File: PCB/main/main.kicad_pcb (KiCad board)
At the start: 2 copper layers, 4 parts, among them J1 Conn_01x33_Female, J2 Conn_01x33_Female, J3 Conn_01x33_Female, J4 Conn_01x33_Female

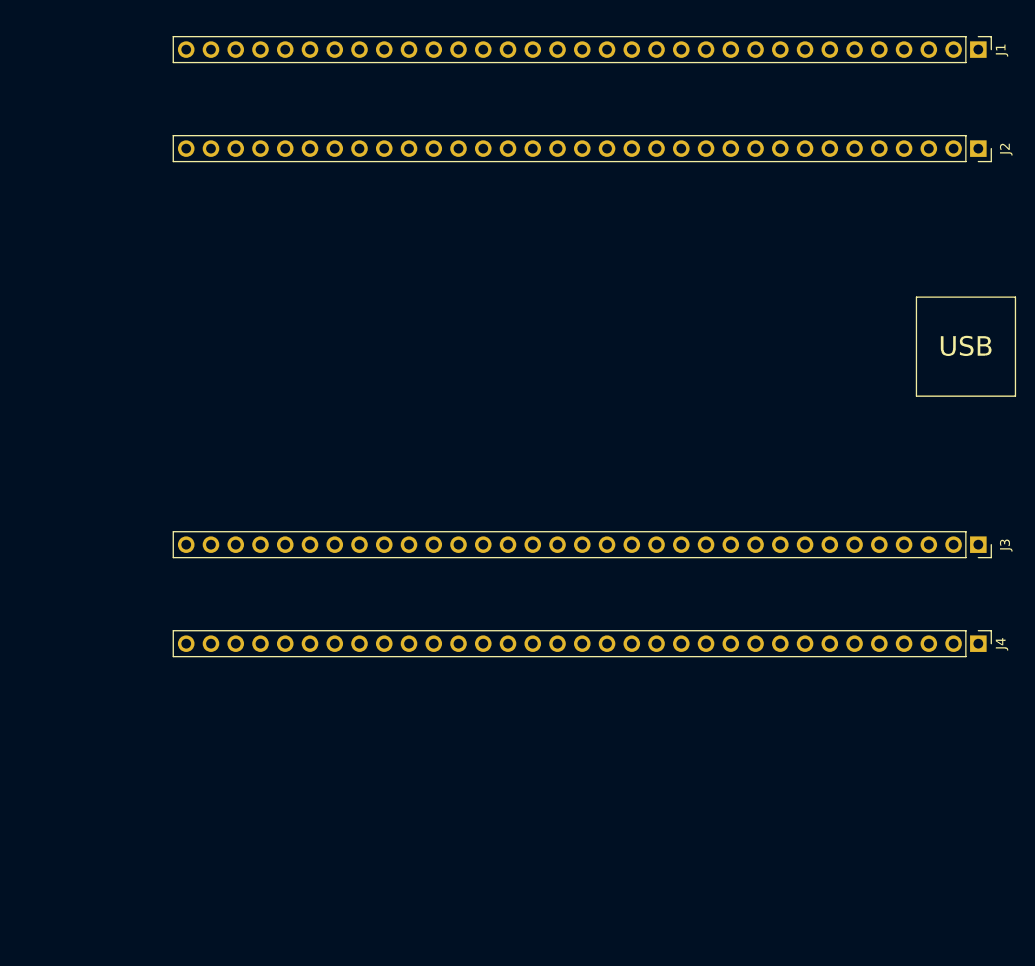
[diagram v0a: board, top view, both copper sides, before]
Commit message: layout started
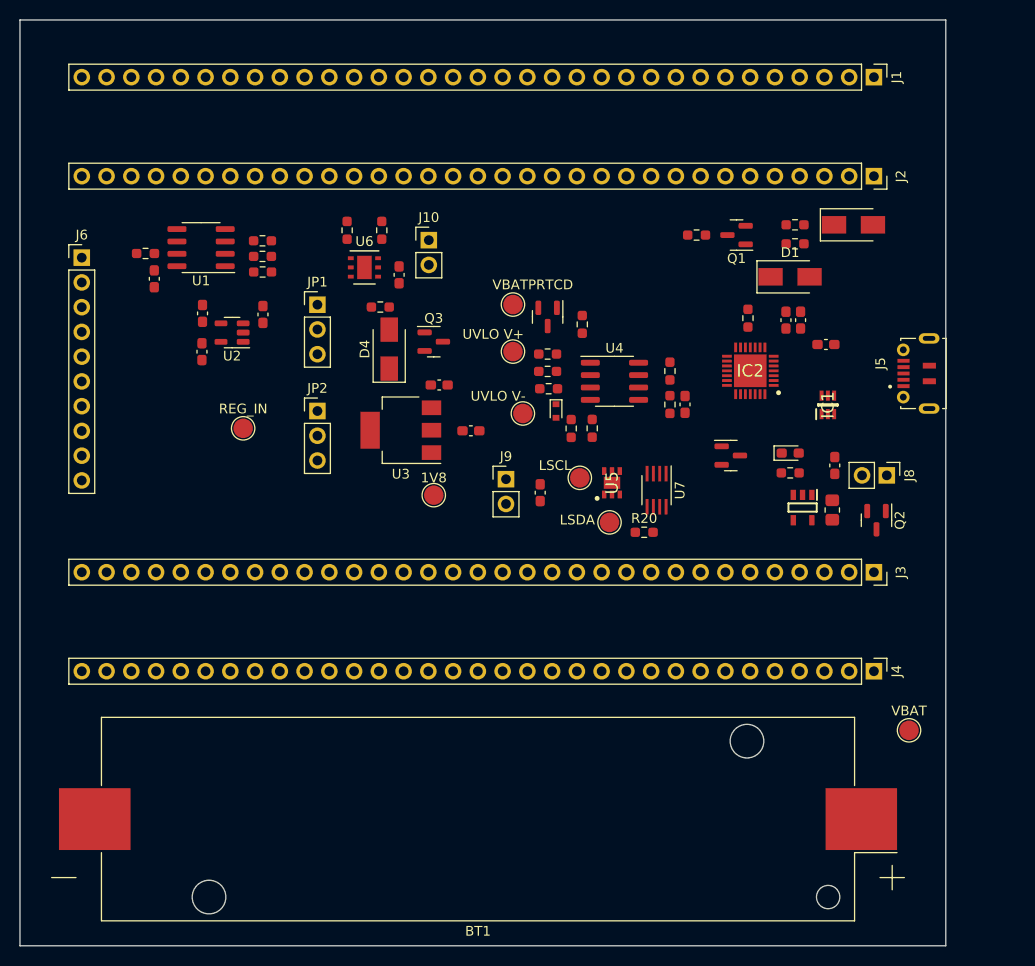
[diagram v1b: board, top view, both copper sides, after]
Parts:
- added 1V8: 1V8, TestPoint:TestPoint_Pad_D2.0mm, F.Cu at (124.5, 111.8)
- added BT1: Battery_Cell, Battery:BatteryHolder_Keystone_1042_1x18650, F.Cu at (129.0, 145.0)
- added C1: 1uF, Capacitor_SMD:C_0603_1608Metric_Pad1.08x0.95mm_HandSolder, F.Cu at (160.6, 93.8)
- added C10: 1uF, Capacitor_SMD:C_0603_1608Metric_Pad1.08x0.95mm_HandSolder, F.Cu at (165.6, 108.7)
- added C11: 1uF, Capacitor_SMD:C_0603_1608Metric_Pad1.08x0.95mm_HandSolder, F.Cu at (150.2, 102.4)
- added C12: 100nF, Capacitor_SMD:C_0603_1608Metric_Pad1.08x0.95mm_HandSolder, F.Cu at (135.4, 111.5)
- added C13: 100nF, Capacitor_SMD:C_0603_1608Metric_Pad1.08x0.95mm_HandSolder, F.Cu at (120.9, 89.2)
- added C2: 100nF, Capacitor_SMD:C_0603_1608Metric_Pad1.08x0.95mm_HandSolder, F.Cu at (162.1, 93.8)
- added C3: 100nF, Capacitor_SMD:C_0603_1608Metric_Pad1.08x0.95mm_HandSolder, F.Cu at (164.7, 96.3)
- added C4: 100nF, Capacitor_SMD:C_0603_1608Metric_Pad1.08x0.95mm_HandSolder, F.Cu at (95.8, 89.6)
- added C5: 1uF, Capacitor_SMD:C_0603_1608Metric_Pad1.08x0.95mm_HandSolder, F.Cu at (106.9, 93.2)
- added C6: 1uF, Capacitor_SMD:C_0603_1608Metric_Pad1.08x0.95mm_HandSolder, F.Cu at (125.0, 100.5)
- added C7: 10nF, Capacitor_SMD:C_0603_1608Metric_Pad1.08x0.95mm_HandSolder, F.Cu at (100.7, 93.1)
- added C8: 1uF, Capacitor_SMD:C_0603_1608Metric_Pad1.08x0.95mm_HandSolder, F.Cu at (128.3, 105.2)
- added C9: 1uF, Capacitor_SMD:C_0603_1608Metric_Pad1.08x0.95mm_HandSolder, F.Cu at (100.7, 97.0)
- added D1: D_Schottky, Diode_SMD:D_SMA, F.Cu at (161.0, 89.4)
- added D2: D_Schottky, Diode_SMD:D_SMA, F.Cu at (167.5, 84.0)
- added D3: CHRG, LED_SMD:LED_0603_1608Metric_Pad1.05x0.95mm_HandSolder, F.Cu at (161.0, 107.4)
- added D4: D_Schottky, Diode_SMD:D_SMA, F.Cu at (119.9, 96.8)
- added D5: D_Zener, Diode_SMD:D_SOD-523, F.Cu at (137.0, 103.1)
- added IC1: SMF05CT1G, SMF05CT1G:SOT65P210X110-6N, F.Cu at (164.9, 102.5)
- added IC2: CP2102-GMR, CP2102-GMR:QFN50P500X500X100-29N-D, F.Cu at (156.9, 99.0)
- added IC3: TP4054-42-SOT25-R, TP4054-42-SOT25-R:SOT95P280X100-5N, F.Cu at (162.3, 113.0)
- added J10: Conn_01x02_Male, Connector_PinHeader_2.54mm:PinHeader_1x02_P2.54mm_Vertical, F.Cu at (124.0, 85.6)
- added J5: USB_B_Micro, MICROXNJ:SHOUHAN_MICROXNJ, F.Cu at (177.0, 99.3)
- added J6: Conn_01x10_Male, Connector_PinHeader_2.54mm:PinHeader_1x10_P2.54mm_Vertical, F.Cu at (88.3, 87.4)
- added J8: Conn_01x02_Male, Connector_PinHeader_2.54mm:PinHeader_1x02_P2.54mm_Vertical, F.Cu at (170.9, 109.7)
- added J9: Conn_01x02_Male, Connector_PinHeader_2.54mm:PinHeader_1x02_P2.54mm_Vertical, F.Cu at (131.9, 110.1)
- added JP1: Jumper_3_Open, Connector_PinHeader_2.54mm:PinHeader_1x03_P2.54mm_Vertical, F.Cu at (112.5, 92.2)
- added JP2: Jumper_3_Open, Connector_PinHeader_2.54mm:PinHeader_1x03_P2.54mm_Vertical, F.Cu at (112.5, 103.1)
- added LSCL: GAS_SCL, TestPoint:TestPoint_Pad_D2.0mm, F.Cu at (139.4, 110.0)
- added LSDA: GAS_SDA, TestPoint:TestPoint_Pad_D2.0mm, F.Cu at (142.5, 114.6)
- added Q1: Q_NMOS_GSD, Package_TO_SOT_SMD:SOT-23, F.Cu at (155.5, 85.1)
- added Q2: Q_PMOS_GSD, Package_TO_SOT_SMD:SOT-23, F.Cu at (169.9, 114.3)
- added Q3: Q_PMOS_GSD, Package_TO_SOT_SMD:SOT-23, F.Cu at (124.5, 96.0)
- added Q4: Q_PMOS_GSD, Package_TO_SOT_SMD:SOT-23, F.Cu at (154.9, 107.7)
- added Q5: Q_PMOS_GSD, Package_TO_SOT_SMD:SOT-23, F.Cu at (136.1, 93.5)
- added R1: 4k7, Resistor_SMD:R_0603_1608Metric_Pad0.98x0.95mm_HandSolder, F.Cu at (161.5, 84.0)
- added R10: 4k7, Resistor_SMD:R_0603_1608Metric_Pad0.98x0.95mm_HandSolder, F.Cu at (119.0, 92.5)
- added R11: 5K1, Resistor_SMD:R_0805_2012Metric_Pad1.20x1.40mm_HandSolder, F.Cu at (165.4, 113.3)
- added R12: 2.2M, Resistor_SMD:R_0603_1608Metric_Pad0.98x0.95mm_HandSolder, F.Cu at (148.7, 99.0)
- added R13: 1M, Resistor_SMD:R_0603_1608Metric_Pad0.98x0.95mm_HandSolder, F.Cu at (148.7, 102.5)
- added R14: 300K, Resistor_SMD:R_0603_1608Metric_Pad0.98x0.95mm_HandSolder, F.Cu at (136.1, 99.1)
- added R15: 1M, Resistor_SMD:R_0603_1608Metric_Pad0.98x0.95mm_HandSolder, F.Cu at (136.1, 97.3)
- added R16: 150, Resistor_SMD:R_0603_1608Metric_Pad0.98x0.95mm_HandSolder, F.Cu at (136.2, 100.8)
- added R17: 100, Resistor_SMD:R_0603_1608Metric_Pad0.98x0.95mm_HandSolder, F.Cu at (138.6, 104.9)
- added R18: 1M, Resistor_SMD:R_0603_1608Metric_Pad0.98x0.95mm_HandSolder, F.Cu at (139.7, 94.2)
- added R19: R, Resistor_SMD:R_0603_1608Metric_Pad0.98x0.95mm_HandSolder, F.Cu at (140.7, 104.9)
- added R2: 4k7, Resistor_SMD:R_0603_1608Metric_Pad0.98x0.95mm_HandSolder, F.Cu at (161.5, 86.0)
- added R20: 4k7, Resistor_SMD:R_0603_1608Metric_Pad0.98x0.95mm_HandSolder, F.Cu at (146.1, 115.6)
- added R22: 4k7, Resistor_SMD:R_0603_1608Metric_Pad0.98x0.95mm_HandSolder, F.Cu at (119.1, 84.6)
- added R23: 4k7, Resistor_SMD:R_0603_1608Metric_Pad0.98x0.95mm_HandSolder, F.Cu at (115.6, 84.6)
- added R3: 4k7, Resistor_SMD:R_0603_1608Metric_Pad0.98x0.95mm_HandSolder, F.Cu at (151.4, 85.1)
- added R4: 4k7, Resistor_SMD:R_0603_1608Metric_Pad0.98x0.95mm_HandSolder, F.Cu at (156.7, 93.6)
- added R5: 4k7, Resistor_SMD:R_0603_1608Metric_Pad0.98x0.95mm_HandSolder, F.Cu at (106.9, 88.9)
- added R6: 4k7, Resistor_SMD:R_0603_1608Metric_Pad0.98x0.95mm_HandSolder, F.Cu at (106.9, 87.3)
- added R7: 4k7, Resistor_SMD:R_0603_1608Metric_Pad0.98x0.95mm_HandSolder, F.Cu at (106.9, 85.7)
- added R8: 4k7, Resistor_SMD:R_0603_1608Metric_Pad0.98x0.95mm_HandSolder, F.Cu at (94.9, 87.0)
- added R9: 510, Resistor_SMD:R_0603_1608Metric_Pad0.98x0.95mm_HandSolder, F.Cu at (161.0, 109.5)
- added REG_IN: REG_IN, TestPoint:TestPoint_Pad_D2.0mm, F.Cu at (104.9, 104.9)
- added U1: CAT24C256, Package_SO:SOIC-8_3.9x4.9mm_P1.27mm, F.Cu at (100.6, 86.4)
- added U2: SGM2007-3.3XN5/TR, Package_TO_SOT_SMD:SOT-23-5, F.Cu at (103.8, 95.1)
- added U3: AMS1117-1.8, Package_TO_SOT_SMD:SOT-223-3_TabPin2, F.Cu at (121.1, 105.1)
- added U4: LM358, Package_SO:SOIC-8_3.9x4.9mm_P1.27mm, F.Cu at (143.0, 100.1)
- added U5: SGP30-2.5k, LIB_SGPC3-2:SON80P245X245X90-7N, F.Cu at (142.7, 110.5)
- added U6: HDC1080, Package_SON:Texas_PWSON-N6, F.Cu at (117.3, 88.4)
- added U7: TXS0102DCT, Package_SO:SSOP-8_2.95x2.8mm_P0.65mm, F.Cu at (147.3, 111.3)
- added UVLO V+: UVLO V+, TestPoint:TestPoint_Pad_D2.0mm, F.Cu at (132.6, 97.0)
- added UVLO V-: UVLO V-, TestPoint:TestPoint_Pad_D2.0mm, F.Cu at (133.6, 103.4)
- added VBAT: VBAT, TestPoint:TestPoint_Pad_D2.0mm, F.Cu at (173.2, 135.9)
- added VBATPRTCD: UVLO_Out, TestPoint:TestPoint_Pad_D2.0mm, F.Cu at (132.6, 92.2)
- moved J1 11.1 mm to (169.6, 68.9)
- moved J2 11.1 mm to (169.6, 79.0)
- moved J3 11.1 mm to (169.6, 119.7)
- moved J4 11.1 mm to (169.6, 129.8)
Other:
- board outline added: 95 x 95 mm
